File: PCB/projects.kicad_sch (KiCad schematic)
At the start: 7 parts, among them SW1 SW_Push, SW2 SW_Push, SW3 SW_Push, SW4 SW_Push, U1 XIAO-RP2040-DIP

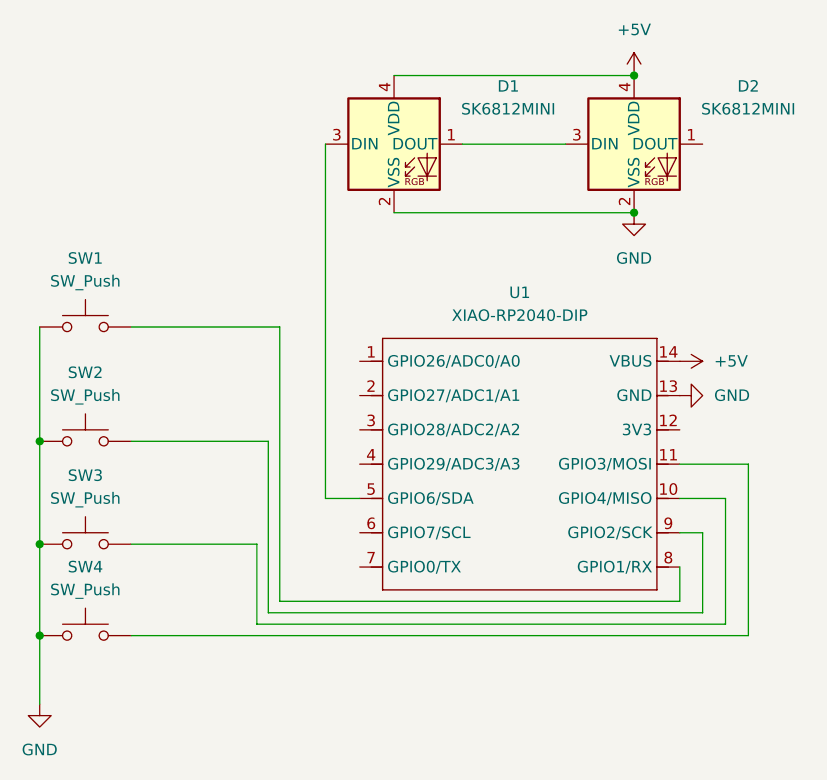
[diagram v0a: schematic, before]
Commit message: Add files via upload
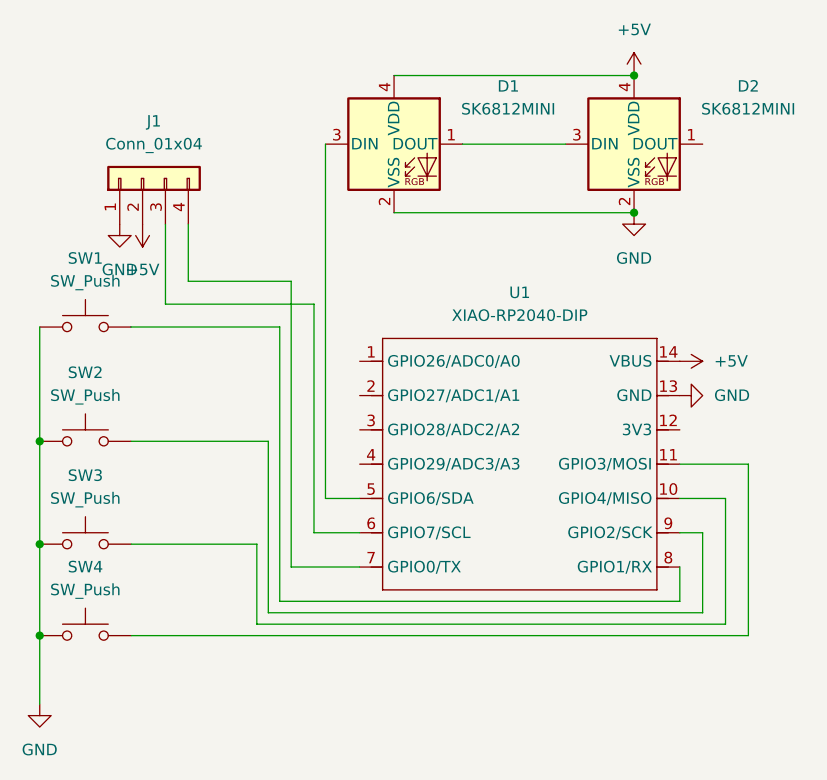
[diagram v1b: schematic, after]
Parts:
- added J1: Conn_01x04, OLED:SSD1306-0.91-OLED-4pin-128x32, symbol Connector_Generic:Conn_01x04
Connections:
- net +5V: now also J1.2 (Pin_2)
- net GND: now also J1.1 (Pin_1)
- net at U1.6 (GPIO7/SCL): now also J1.3 (Pin_3)
- net at U1.7 (GPIO0/TX): now also J1.4 (Pin_4)
